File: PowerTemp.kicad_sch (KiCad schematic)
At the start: 45 parts, among them U28 LMV321, U33 74HC123, U6 74HC123, U63 LMV321, U64 74HC4051, U70 LMV321, U71 LMV321

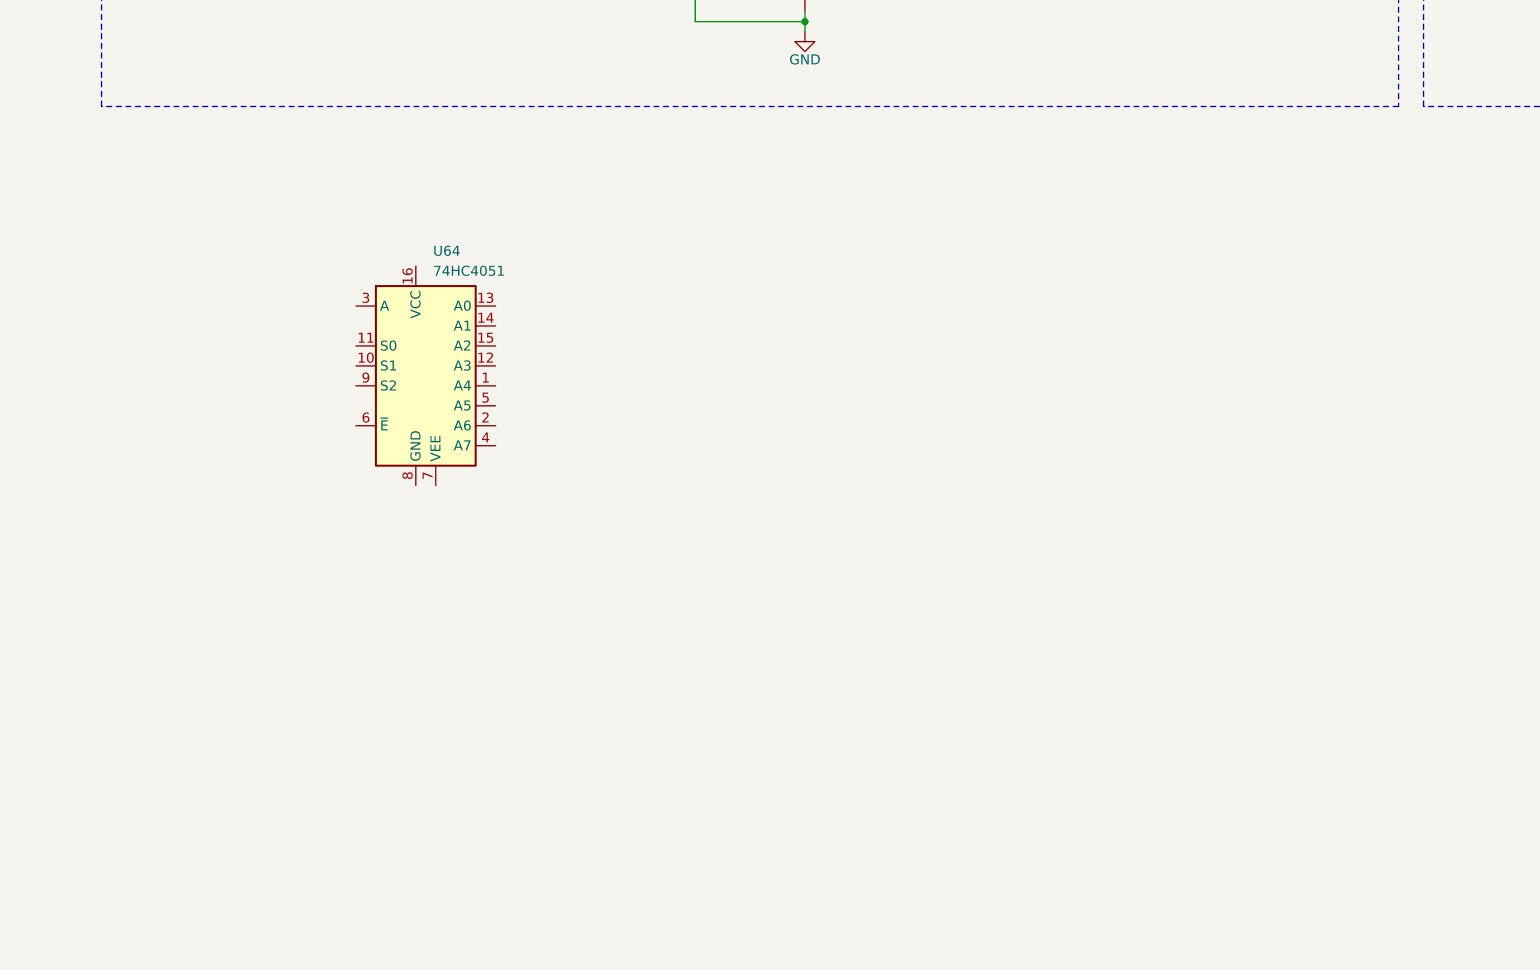
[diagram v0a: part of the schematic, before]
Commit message: Добавления: Расставил все на плате
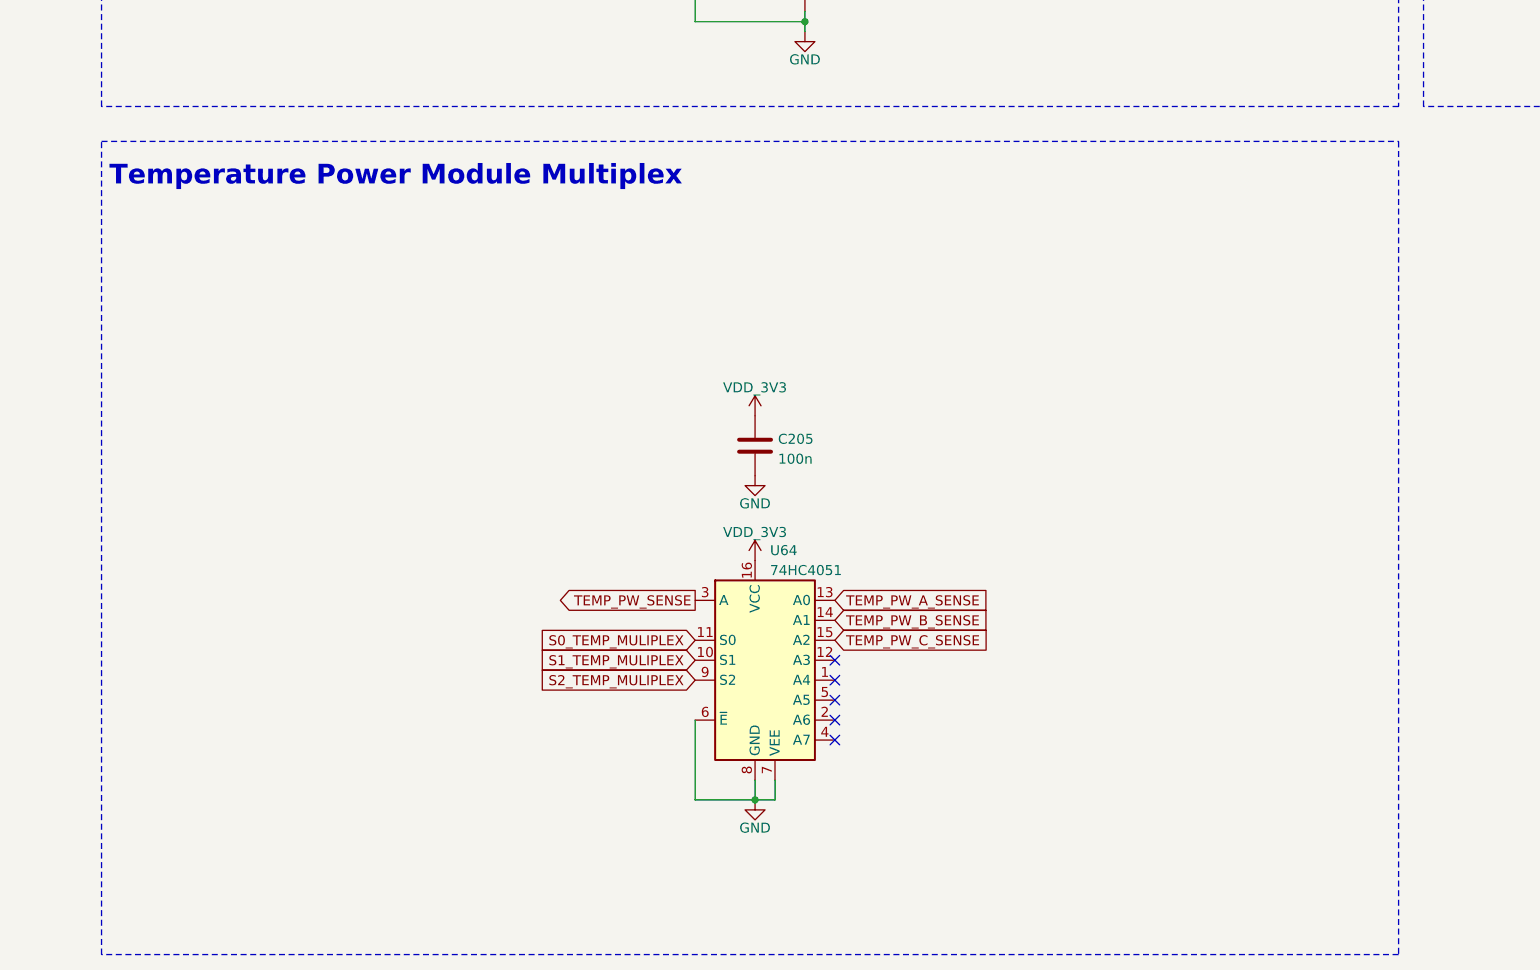
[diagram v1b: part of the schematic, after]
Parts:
- added C205: 100n, Capacitor_SMD:C_0603_1608Metric, symbol Device:C
- U64: footprint (none) -> Package_SO:SOIC-16_3.9x9.9mm_P1.27mm
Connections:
- net GND: now also U64.6 (~{E}), U64.7 (VEE), U64.8 (GND), C205.1
- net TEMP_PW_A_SENSE: now also U64.13 (A0)
- net TEMP_PW_B_SENSE: now also U64.14 (A1)
- net TEMP_PW_C_SENSE: now also U64.15 (A2)
- net VDD_3V3: now also U64.16 (VCC), C205.2
- net S1_TEMP_MULIPLEX: now reaches U64.10 (S1)
- net S0_TEMP_MULIPLEX: now reaches U64.11 (S0)
- net TEMP_PW_SENSE: now reaches U64.3 (A)
- net S2_TEMP_MULIPLEX: now reaches U64.9 (S2)
- no-connect marks 4 -> 9
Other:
- note added: "Temperature Power Module Multiplex"
- moved on the sheet: U64
